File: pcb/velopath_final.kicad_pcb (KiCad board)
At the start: 2 copper layers, 15.5 x 47 mm, 64 parts, among them J1 charger, J2 battery, J3 control, J4 gnd, J5 ESC_power, J6 control, J7 gnd, P2 SWD, Q6 2SJ168, SW1 Push_Button, U1 LIS3MDL, U3 STM32F103RGTx, Y2 8MHz

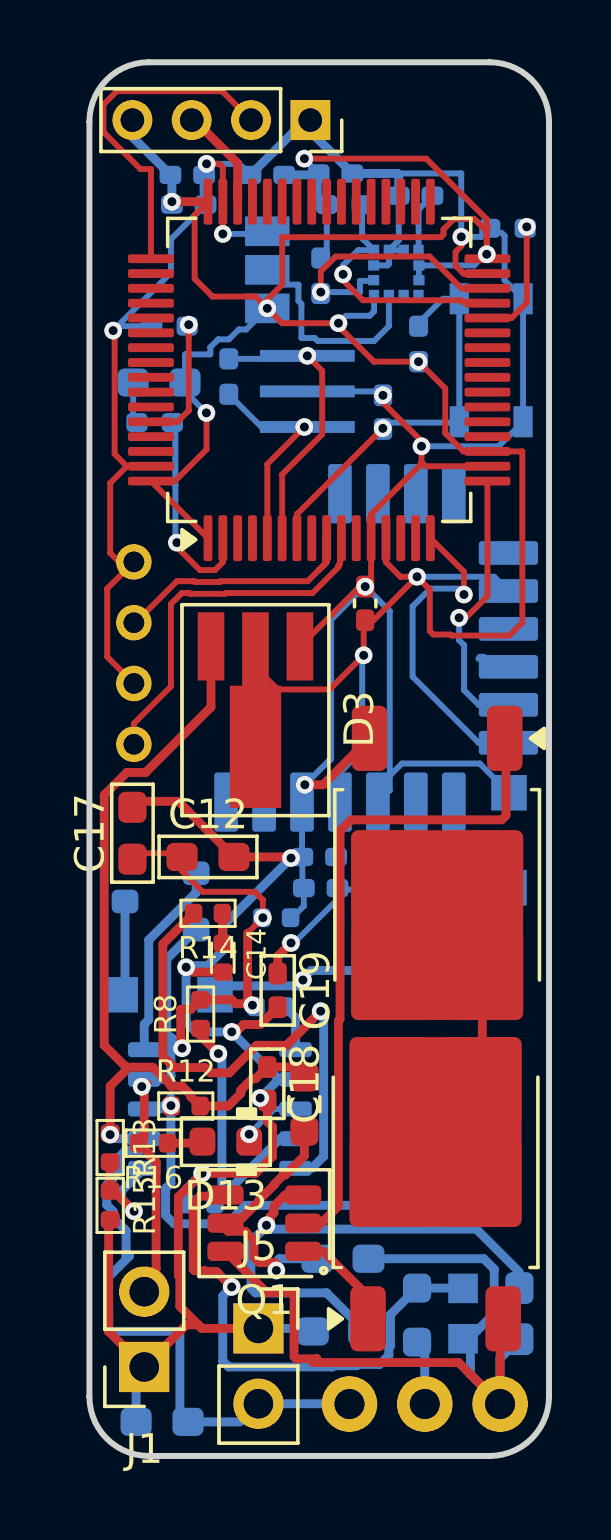
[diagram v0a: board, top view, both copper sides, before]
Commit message: Sync repository with current project state
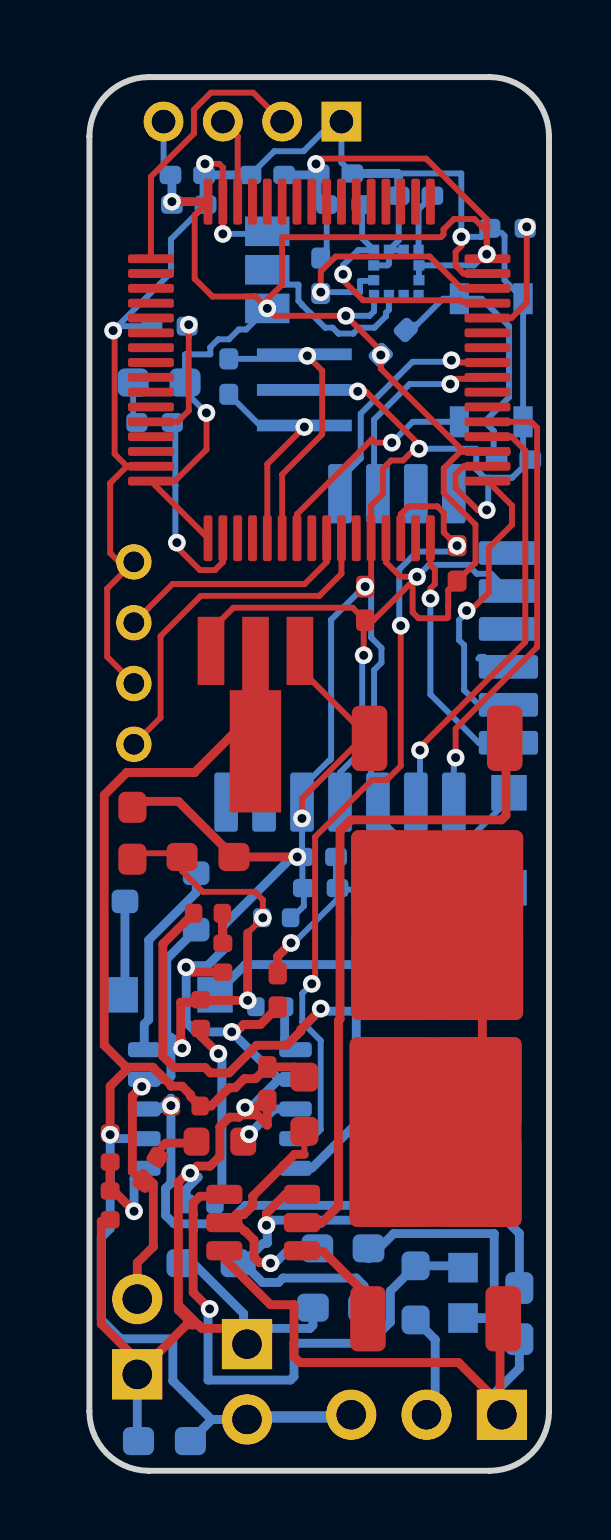
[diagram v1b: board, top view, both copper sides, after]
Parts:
- added R17: 10 kOm, Resistor_SMD:R_0402_1005Metric_Pad0.72x0.64mm_HandSolder, F.Cu at (32.4, 39.9)
- added R18: 2k, Resistor_SMD:R_0603_1608Metric_Pad0.98x0.95mm_HandSolder, B.Cu at (24.0, 63.5)
- ?: renamed from C26; value C,IEC -> 10nF
- C18, C19: value 10 uF -> 22 uF
- C23, C24: value C,IEC -> 100nF
- C25: value C,IEC -> 10nF
- J2: footprint PCM_SparkFun-Connector:1x03_P2.54mm -> Connector_PinSocket_2.54mm:PinSocket_1x03_P2.54mm_Vertical
- Q1: value ~ -> HY2122-AB1B
- Q2, Q3: value ~ -> N-MOSFET 30V logic-level
- R10, R9: value R,IEC -> 470R
- U7: renamed from D7; value ~ -> CN3765
- moved C1 4.68 mm to (34.3, 36.4), turned to 0 degrees
- moved P2 1.05 mm to (28.5, 25.0)
- moved R16 0.91 mm to (22.1, 60.4), turned to -120 degrees
- moved R2 0.85 mm to (30.2, 32.5), turned to 45 degrees
- moved ? 0.80 mm to (28.4, 65.0)
- moved R9 0.75 mm to (31.0, 64.5)
- moved C23 0.70 mm to (32.6, 64.5)
- moved J5 0.66 mm to (25.3, 66.2)
- moved C15 0.65 mm to (22.5, 69.5)
- moved R1 0.52 mm to (30.2, 50.1)
- moved D1 0.50 mm to (30.6, 51.4)
- moved J2 0.36 mm to (33.9, 68.6), turned to -90 degrees
- moved C24 0.35 mm to (28.6, 63.0)
- moved J1 0.34 mm to (21.6, 67.2)
- moved D13 0.20 mm to (24.4, 59.4)
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- renumbered R8 to ?, R17 to ?
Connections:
- net P- renamed GND
- D3 pad 2: +3.3V -> B+
- D3 pad 3: B+ -> +3.3V
- U3 pad 14: unconnected-(U3-PA0-Pad14) -> chrg_done
- U3 pad 20: unconnected-(U3-PA4-Pad20) -> nReset
- U3 pad 21: unconnected-(U3-PA5-Pad21) -> Link
- U3 pad 24: unconnected-(U3-PC4-Pad24) -> nWake
- U3 pad 25: unconnected-(U3-PC5-Pad25) -> nReload
- U6 pad 1: unconnected-(U6-nReload-Pad1) -> nReload
- U6 pad 11: unconnected-(U6-Link-Pad11) -> Link
- U6 pad 12: unconnected-(U6-nReset-Pad12) -> nReset
- U6 pad 2: unconnected-(U6-nWake-Pad2) -> nWake
- U7 pad 4: Net-(R17--) -> chrg_done
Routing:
- net chrg_done: track 0.00 -> 27.9 mm, vias 0 -> 3
- net Link: track 0.00 -> 15.5 mm, vias 0 -> 1
- net GND: track 154.1 -> 169.3 mm, vias 13 -> 14
- net nReset: track 0.00 -> 14.9 mm, vias 0 -> 1
- net nReload: track 0.00 -> 8.18 mm, vias 0 -> 1
- net B+: track 47.2 -> 55.1 mm
- net nWake: track 0.00 -> 7.18 mm, vias 0 -> 1
- net RESET: track 13.6 -> 17.8 mm
- net Net-(R17--): track 10.3 -> 6.14 mm
- net SWDCLK: track 11.6 -> 9.24 mm
- net BTX: track 11.1 -> 8.70 mm
- net Net-(R14--): track 17.7 -> 19.5 mm
- net +3.3V: track 102.4 -> 100.7 mm
- net Vibro_R: track 9.39 -> 8.25 mm
- net Net-(JP1-B): track 7.78 -> 6.65 mm
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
